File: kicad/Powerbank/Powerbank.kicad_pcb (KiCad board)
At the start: 2 copper layers, 90 x 60 mm, 166 parts, among them IC1 BQ4050RSMR, IC2 SN74LVC1G14DSFR, IC3 SN74LVC1G08DSFR, IC4 BQ25703ARSNT, IC5 TPD6S300ARUKR, IC6 W25Q80DVSNIG, J1 USB_C_Receptacle, J2 USB_A, J3 Conn_01x02_Male, J4 Conn_01x05_Male, J5 Conn_01x08_Male, J6 Conn_01x04_Male, Q1 Q_NMOS_GDS, Q2 Q_PMOS_GDS, Q3 Q_NMOS_GDS, Q4 Q_NMOS_GDS, Q5 Q_NMOS_GDS, Q6 Q_NMOS_GDS, Q7 Q_NMOS_GDS, Q8 Q_PMOS_GDS, SW1 SW_DIP_x01, U1 TPS65988DH

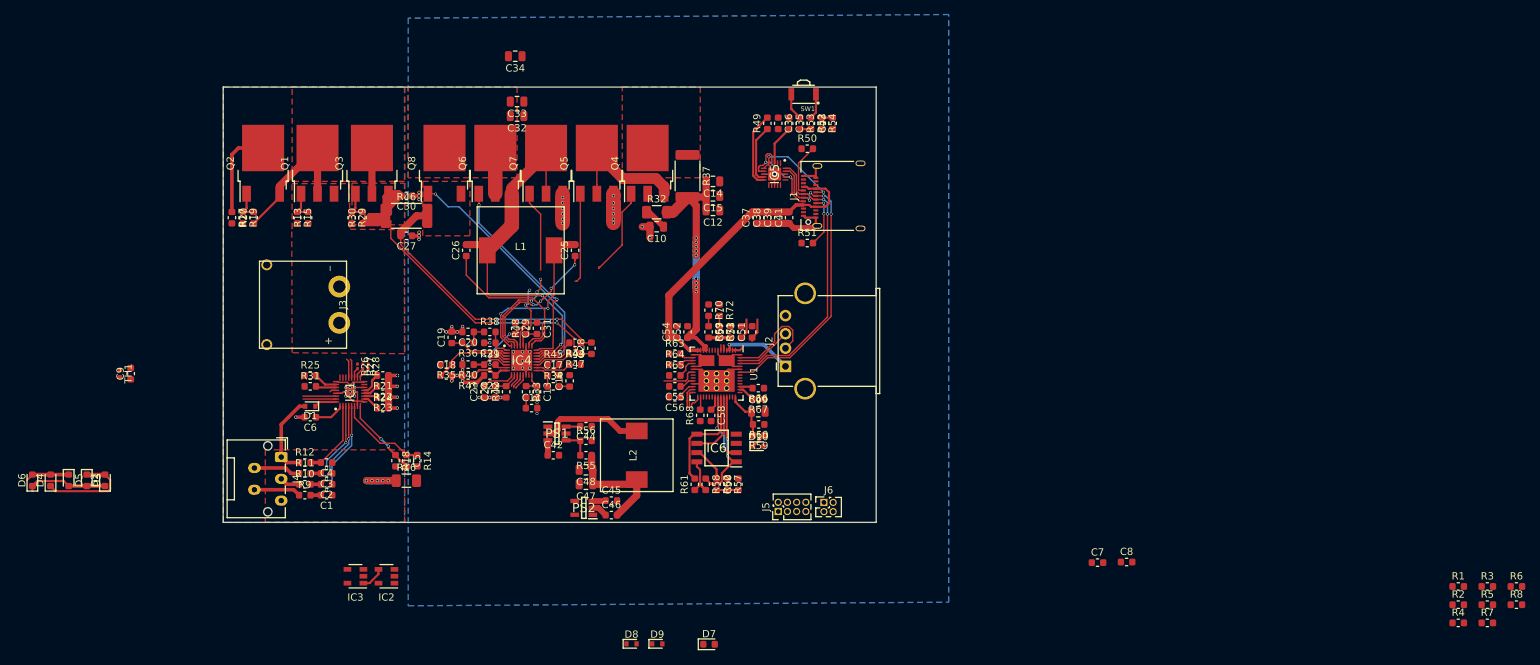
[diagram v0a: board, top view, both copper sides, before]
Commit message: First routing finished, correcting DRC warnings
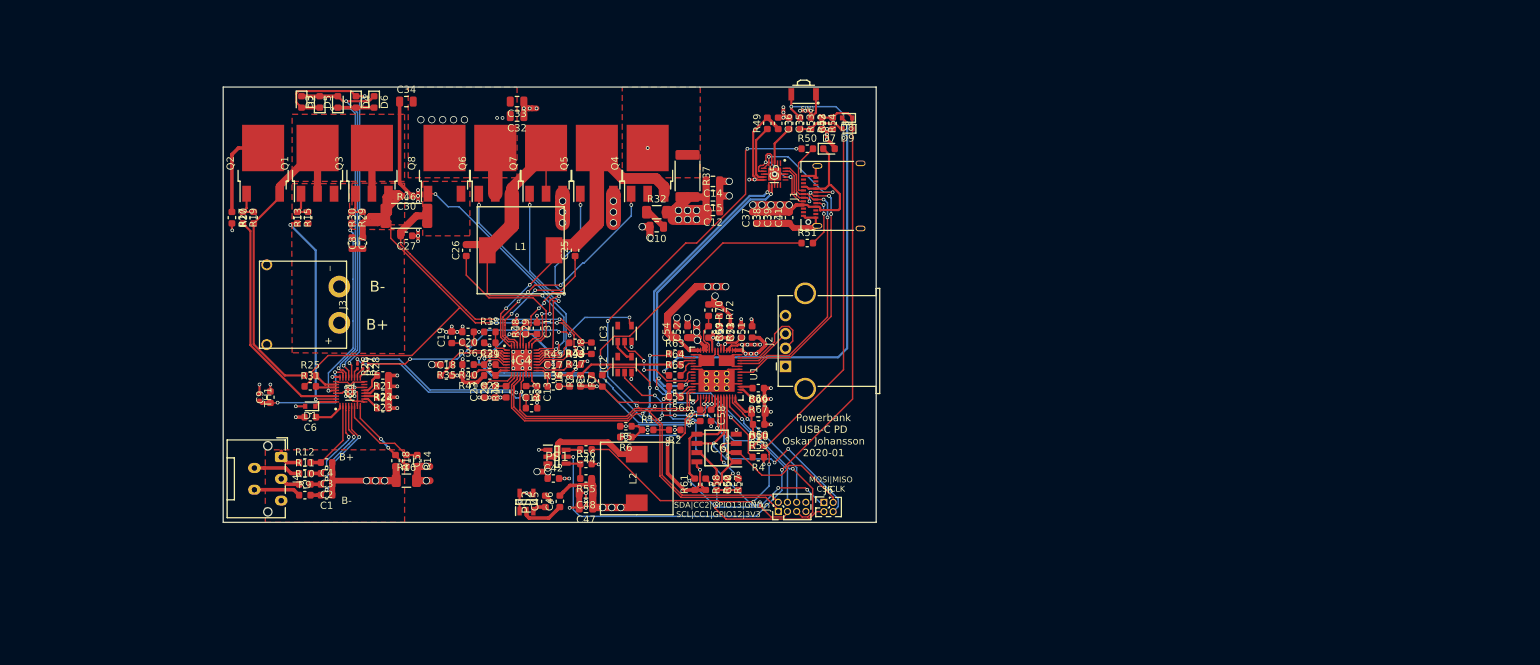
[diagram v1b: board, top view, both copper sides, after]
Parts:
- moved R8 132.6 mm to (149.2, 110.5), turned to 90 degrees
- moved R3 126.7 mm to (150.8, 110.5), turned to 90 degrees
- moved R7 126.5 mm to (152.2, 110.5), turned to 90 degrees
- moved R6 124.5 mm to (155.5, 118.2), turned to 180 degrees
- moved R5 121.3 mm to (155.5, 116.8), turned to 180 degrees
- moved C8 114.1 mm to (119.2, 91.5), turned to 90 degrees
- moved R1 113.8 mm to (158.5, 117.2)
- moved C7 111.8 mm to (117.8, 91.5), turned to 270 degrees
- moved R2 110.6 mm to (162.2, 117.2), turned to 180 degrees
- moved R4 99.1 mm to (173.8, 121.0), turned to 180 degrees
- moved D8 78.3 mm to (186.0, 74.2), turned to 180 degrees
- moved D9 75.7 mm to (186.1, 75.8), turned to 180 degrees
- moved D7 70.3 mm to (183.5, 78.5)
- moved D6 70.3 mm to (120.8, 72.0), turned to 270 degrees
- moved D4 67.0 mm to (118.3, 72.0), turned to 270 degrees
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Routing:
- net SCL_1: track 5.37 -> 143.2 mm, vias 0 -> 8
- net SYS: track 17.4 -> 152.3 mm, vias 0 -> 13
- net SDA_1: track 4.74 -> 134.7 mm, vias 0 -> 4
- net SYS_EN: track 1.50 -> 99.0 mm, vias 0 -> 2
- net PD_LDO_3V3: track 18.9 -> 116.2 mm, vias 0 -> 11
- net SW: track 3.71 -> 96.1 mm, vias 0 -> 4
- net GND: track 61.5 -> 150.9 mm, vias 46 -> 79
- net CC1: track 2.05 -> 73.4 mm, vias 0 -> 5
- net +3V3: track 3.49 -> 72.4 mm, vias 0 -> 2
- net CC2: track 2.51 -> 66.2 mm, vias 0 -> 2
- net SRC_EVT: track 0.00 -> 59.6 mm, vias 0 -> 2
- net PP_HV: track 40.4 -> 94.9 mm
- net PROCHOT: track 1.91 -> 44.0 mm, vias 0 -> 3
- net Net-(D4-Pad2): track 6.03 -> 47.5 mm, vias 0 -> 2
- net Net-(C20-Pad1): track 2.93 -> 43.9 mm, vias 0 -> 2
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- added copper zone on GND.Cu, net -BATT
- added copper zone on POWER.Cu, net CELL4
- added copper zone on GND.Cu, net GND
- removed copper zone on B.Cu, net -BATT
- removed copper zone on B.Cu, net GND
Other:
- copper layers 2 -> 4
- rule trace_min: 0.2 -> 0.1
- rule via_min_size: 0.4 -> 0.5
- board text added: "B+"
- board text added: "B-"
- board text added: "MOSI|MISO CS|CLK"
- board text added: "Powerbank USB-C PD Oskar Johansson 2020-01"
- board text added: "SDA|CC2|GPIO13|GND SCL|CC1|GPIO12|3V3"
